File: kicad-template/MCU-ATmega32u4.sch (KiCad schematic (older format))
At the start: 25 parts, among them J1 ICSP, SW1 SW_PUSH, T5 ICSP_Test, U1 ATMEGA32U4-MU, X1 16Mhz-18pF

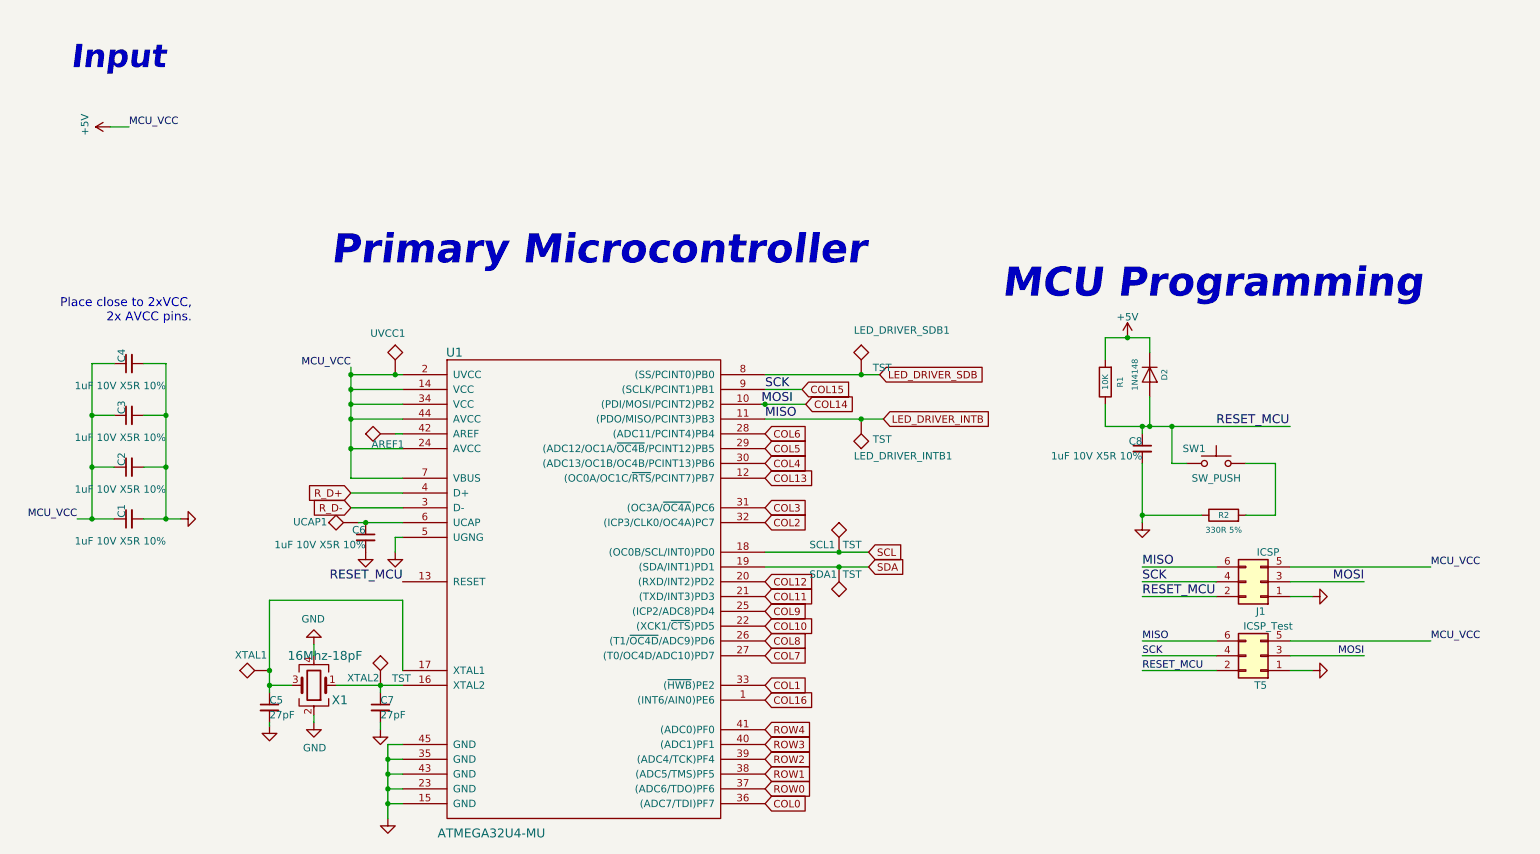
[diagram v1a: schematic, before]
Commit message: snapshot changes
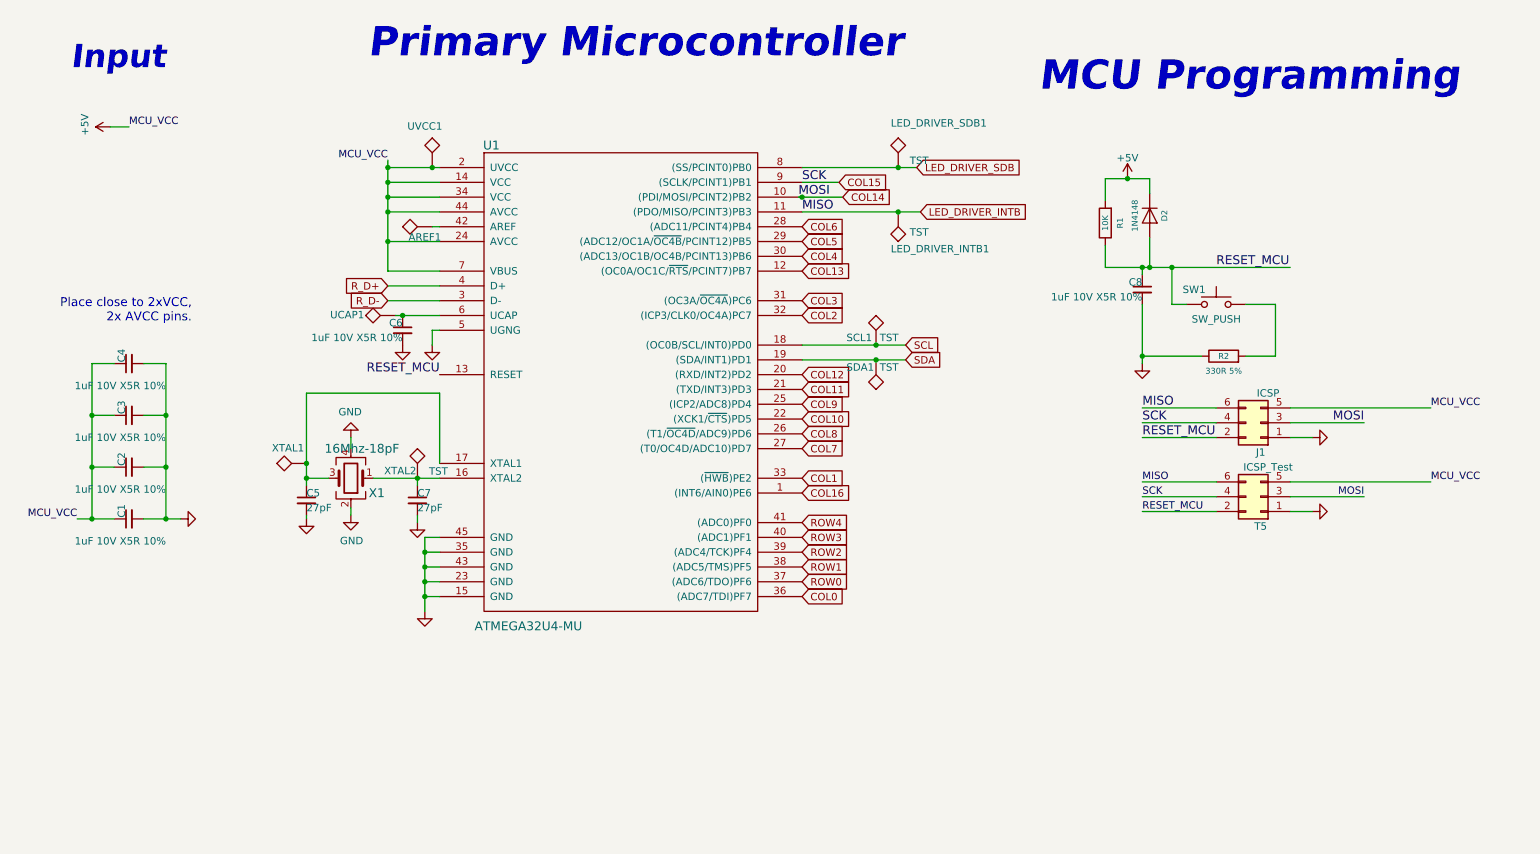
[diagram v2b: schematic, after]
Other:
- moved on the sheet: AREF1, C5, C6, C7, C8, D2, J1, LED_DRIVER_INTB1, LED_DRIVER_SDB1, R1, R2, SCL1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
